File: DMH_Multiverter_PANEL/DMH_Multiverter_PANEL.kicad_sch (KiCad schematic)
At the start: 5 parts, among them J0 Panel_GND_Solder_Wire_Pad

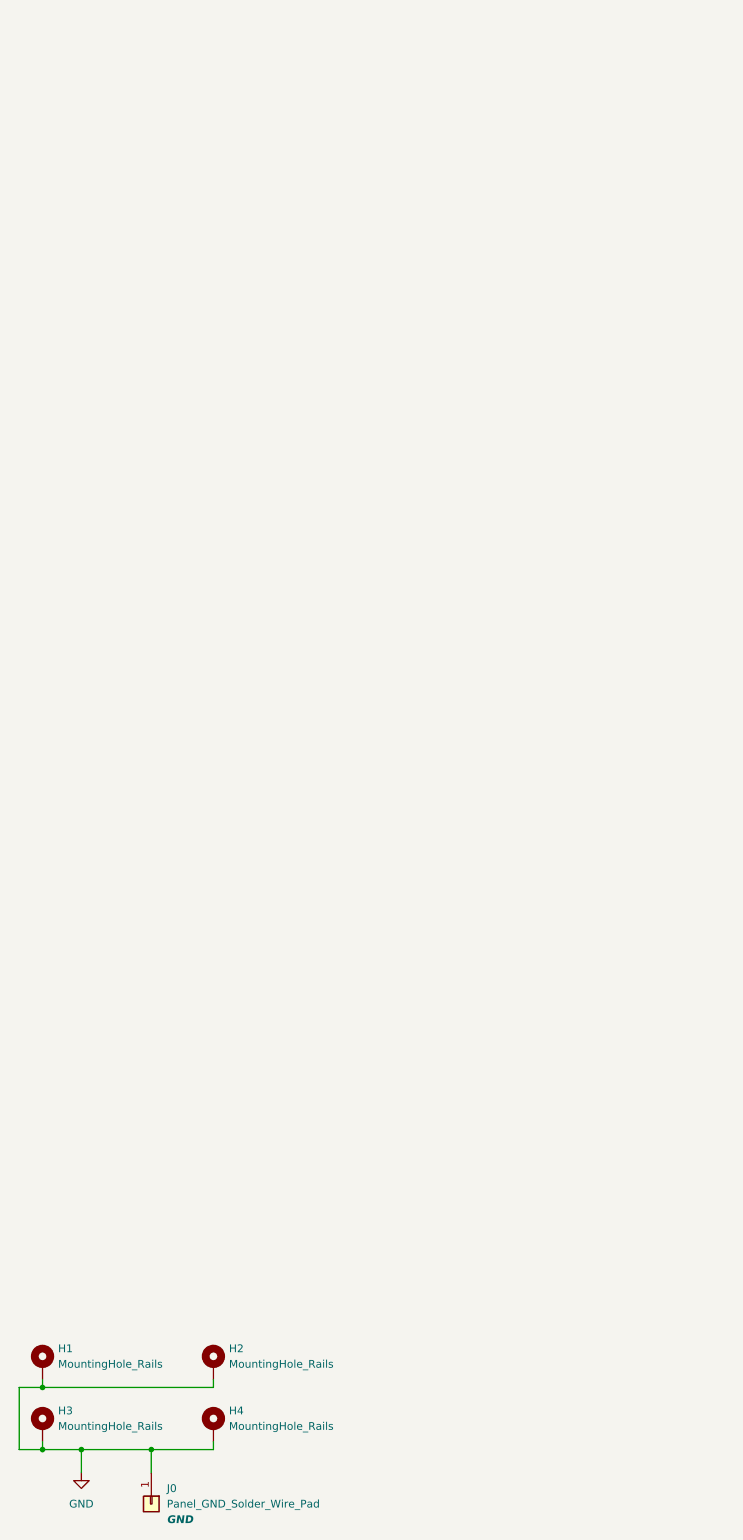
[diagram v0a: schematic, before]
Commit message: Panel ready
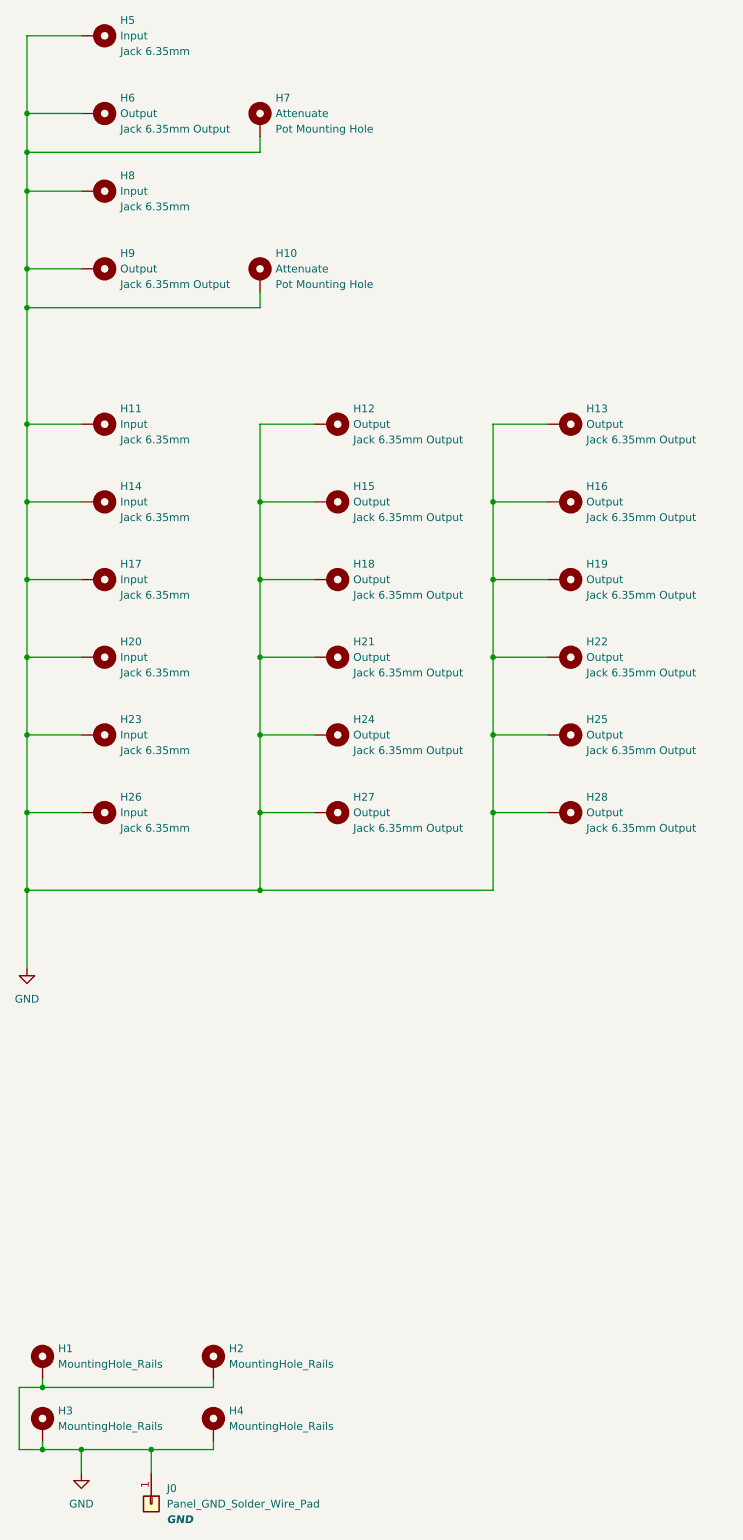
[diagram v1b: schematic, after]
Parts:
- added H10, H7: Attenuate, SynthStuff:Pot_Cutout_Small_attv, symbol SynthStuff:MountingHole_Pot
- added H11, H14, H17, H20, H23, H26, H5, H8: Input, SynthStuff:Jack_6.35mm_Cutout_v3, symbol SynthStuff:MountingHole_Jack6.35mm_v2
- added H12, H13, H15, H16, H18, H19, H21, H22, H24, H25, H27, H28, H6, H9: Output, SynthStuff:Jack_6.35mm_Cutout_Output_v6, symbol SynthStuff:MountingHole_Jack6.35mm_Output_v2
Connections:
- net GND: now also H10.1, H11.1, H12.1, H13.1, H14.1, H15.1, H16.1, H17.1, H18.1, H19.1, H20.1, H21.1, H22.1, H23.1, H24.1, H25.1, H26.1, H27.1, H28.1, H5.1, H6.1, H7.1, H8.1, H9.1

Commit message: Generated BoM
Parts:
- H10, H7: now in the parts list
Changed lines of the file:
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@@
 		(unit 1)
 		(exclude_from_sim yes)
-		(in_bom no)
+		(in_bom yes)
 		(on_board yes)
 		(dnp no)
@@
 		(unit 1)
 		(exclude_from_sim yes)
-		(in_bom no)
-		(on_board yes)
-		(dnp no)
+		(in_bom yes)
+		(on_board yes)
+		(dnp no)

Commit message: Sync libs
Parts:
- H10, H7: footprint SynthStuff:Pot_Cutout_Small_attv -> SynthStuff:Pot_Cutout_Small_attv_P110KH1
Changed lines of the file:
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@@
 			)
 		)
-		(property "Footprint" "SynthStuff:Pot_Cutout_Small_attv"
+		(property "Footprint" "SynthStuff:Pot_Cutout_Small_attv_P110KH1"
 			(at 63.5 77.47 0)
 			(effects
@@
 			)
 		)
-		(property "Footprint" "SynthStuff:Pot_Cutout_Small_attv"
+		(property "Footprint" "SynthStuff:Pot_Cutout_Small_attv_P110KH1"
 			(at 63.5 52.07 0)
 			(effects
